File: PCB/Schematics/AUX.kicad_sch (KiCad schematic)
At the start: 31 parts, among them J14 Conn_01x02, J17 Conn_01x02, J18 Conn_01x02, J19 Conn_01x02, J20 Conn_01x03, J21 EXP1, J22 EXP2, J23 5015_Connector, J24 3010_Connector, J25 Conn_01x02, J26 Conn_01x02, Q2 IRLB8721PBF, Q3 IRLB8721PBF

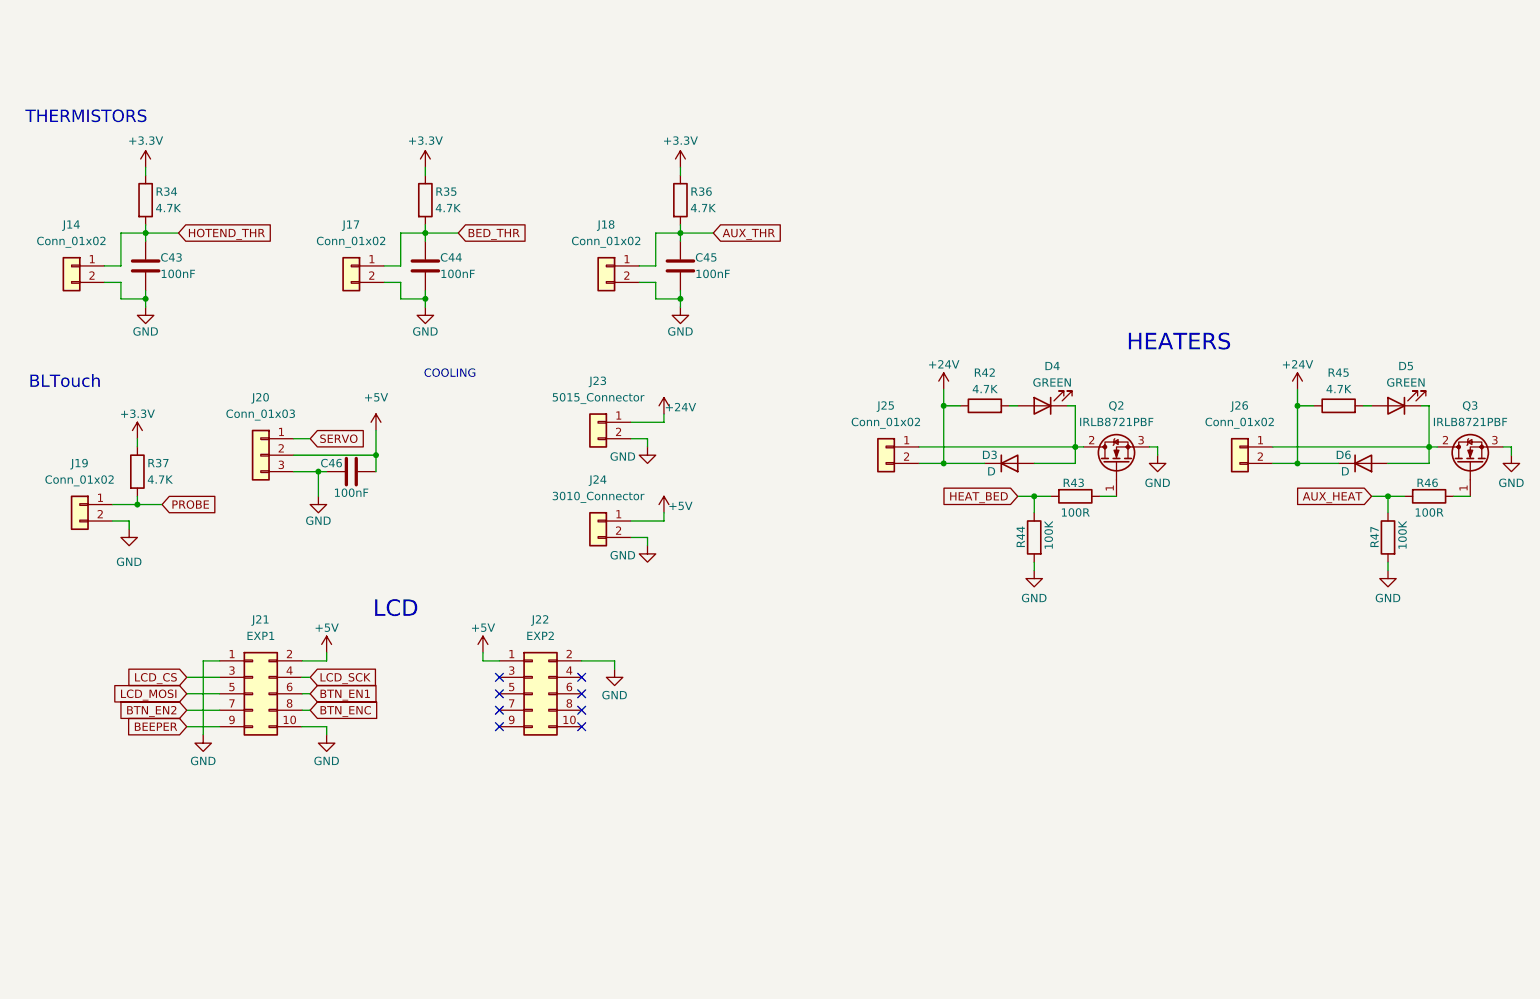
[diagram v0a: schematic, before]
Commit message: Add changes
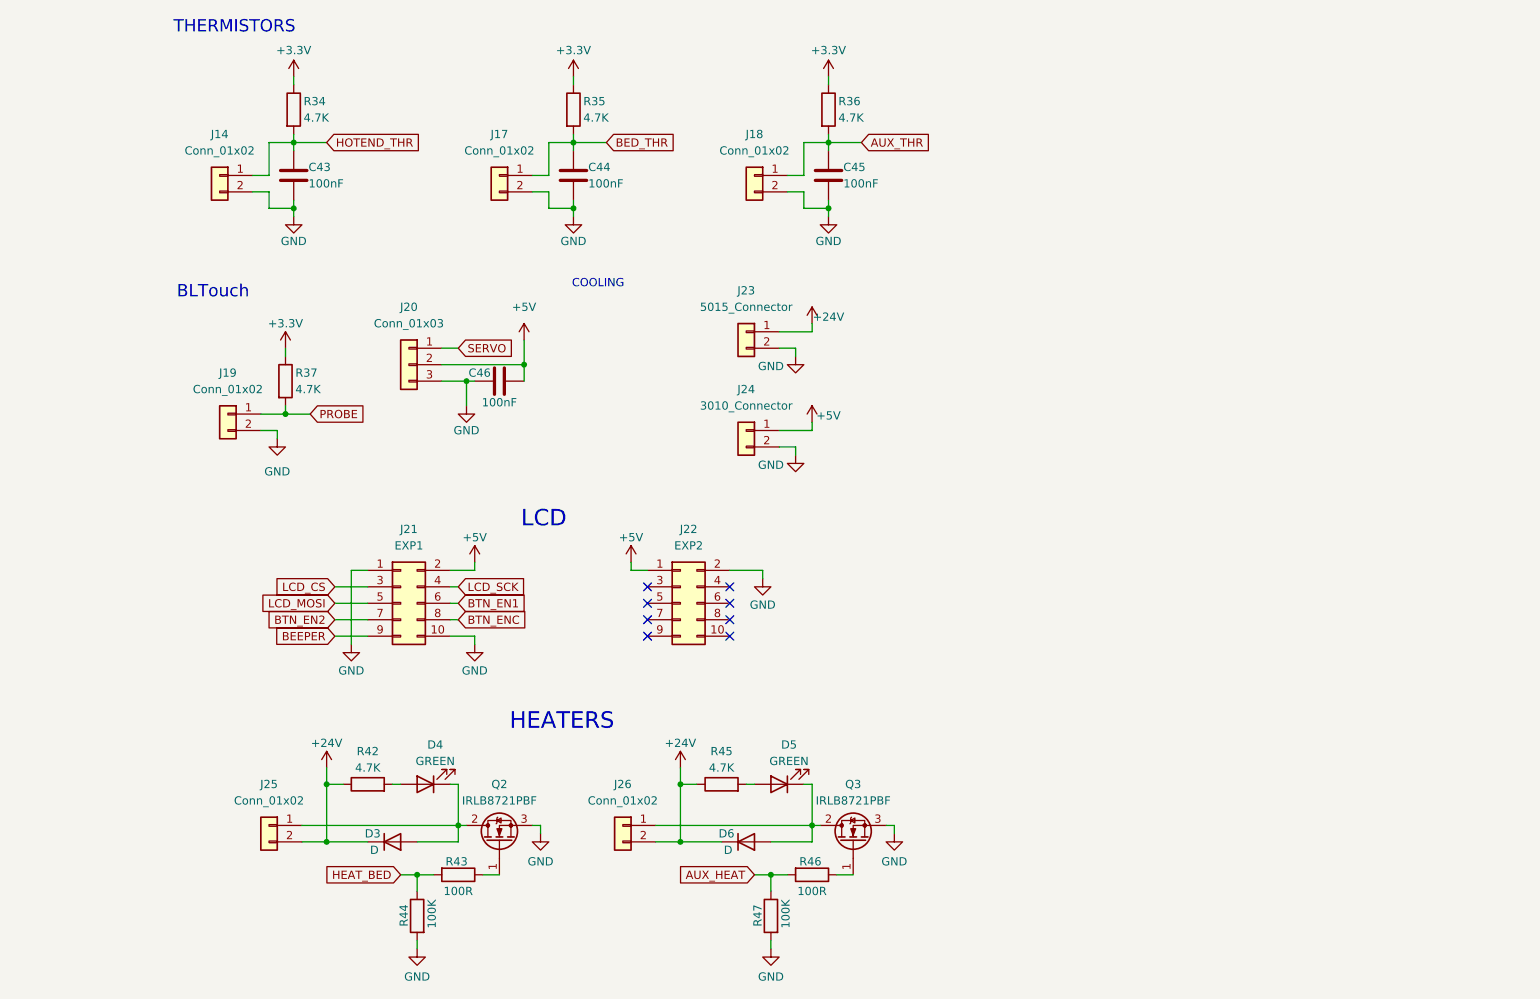
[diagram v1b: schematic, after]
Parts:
- J21, J22: footprint Connector_IDC:IDC-Header_2x05_P2.54mm_Vertical_SMD -> Connector_IDC:IDC-Header_2x05_P2.54mm_Vertical
- Q2, Q3: footprint Package_TO_SOT_THT:TO-220-3_Vertical -> AOD4184A:TO252_AOS
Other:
- moved on the sheet: C43, C44, C45, C46, D3, D4, D5, D6, J14, J17, J18, J19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
